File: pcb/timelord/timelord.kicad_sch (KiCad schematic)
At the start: 37 parts, among them J1 GPIO, J2 BCKP_PWR, J3 OLED, J4 EXTERNAL, J5 SMA, J6 SMA, Q1 BC846, Q2 BC846, U1 NEO-F10T, U2 DS3232M

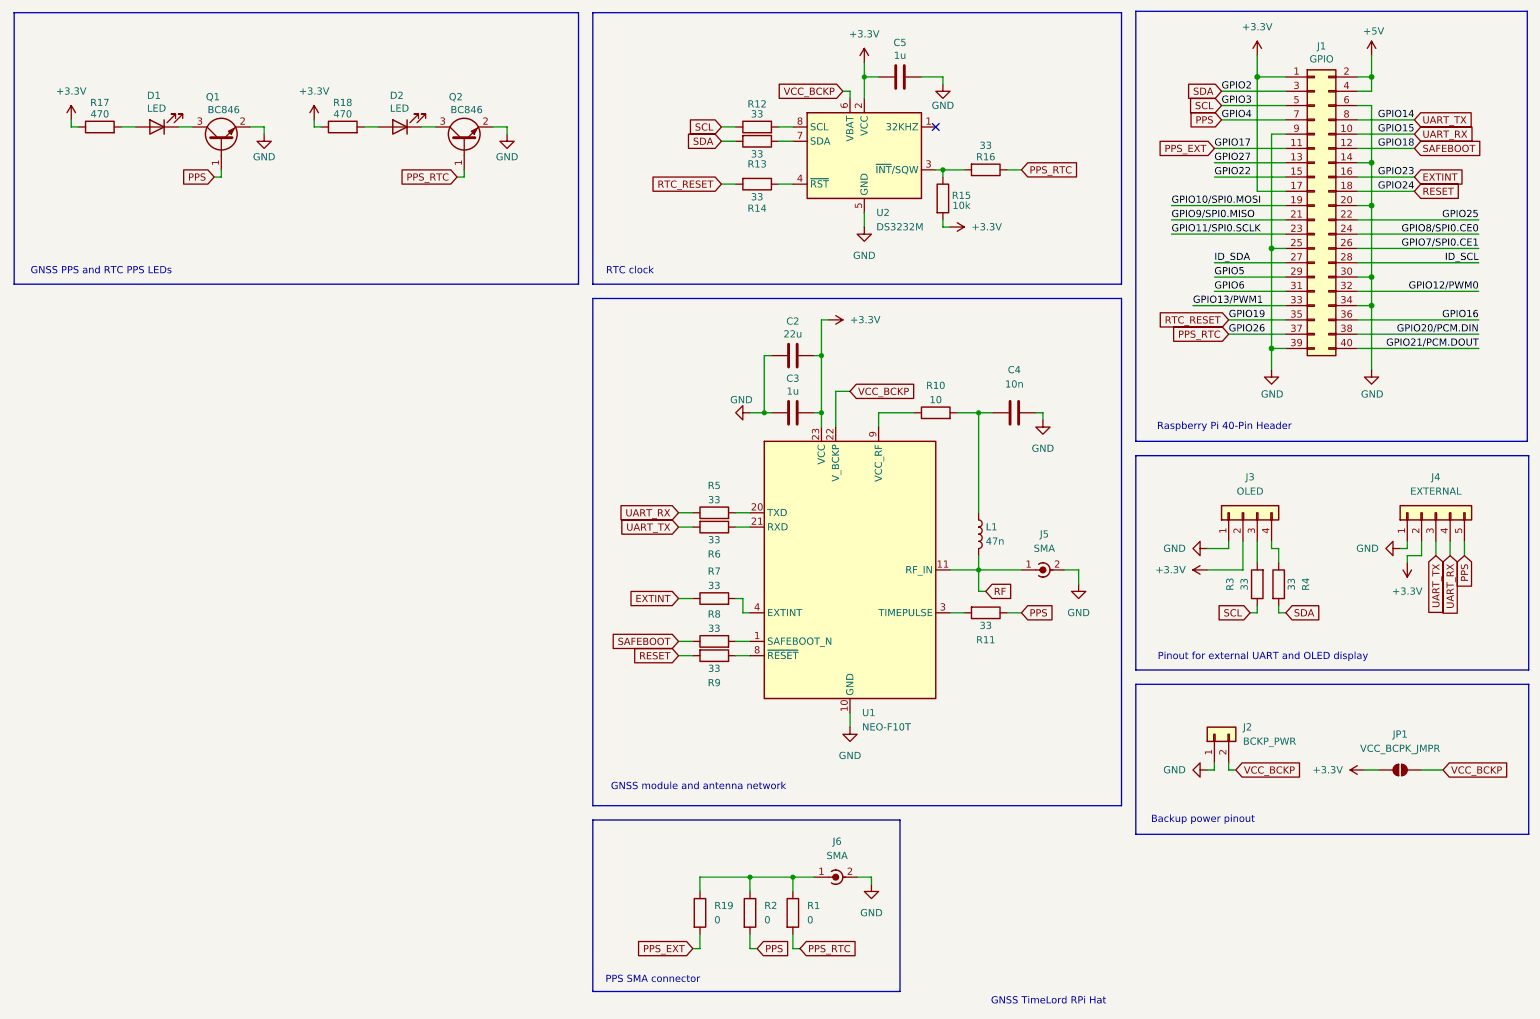
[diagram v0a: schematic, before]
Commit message: Changes
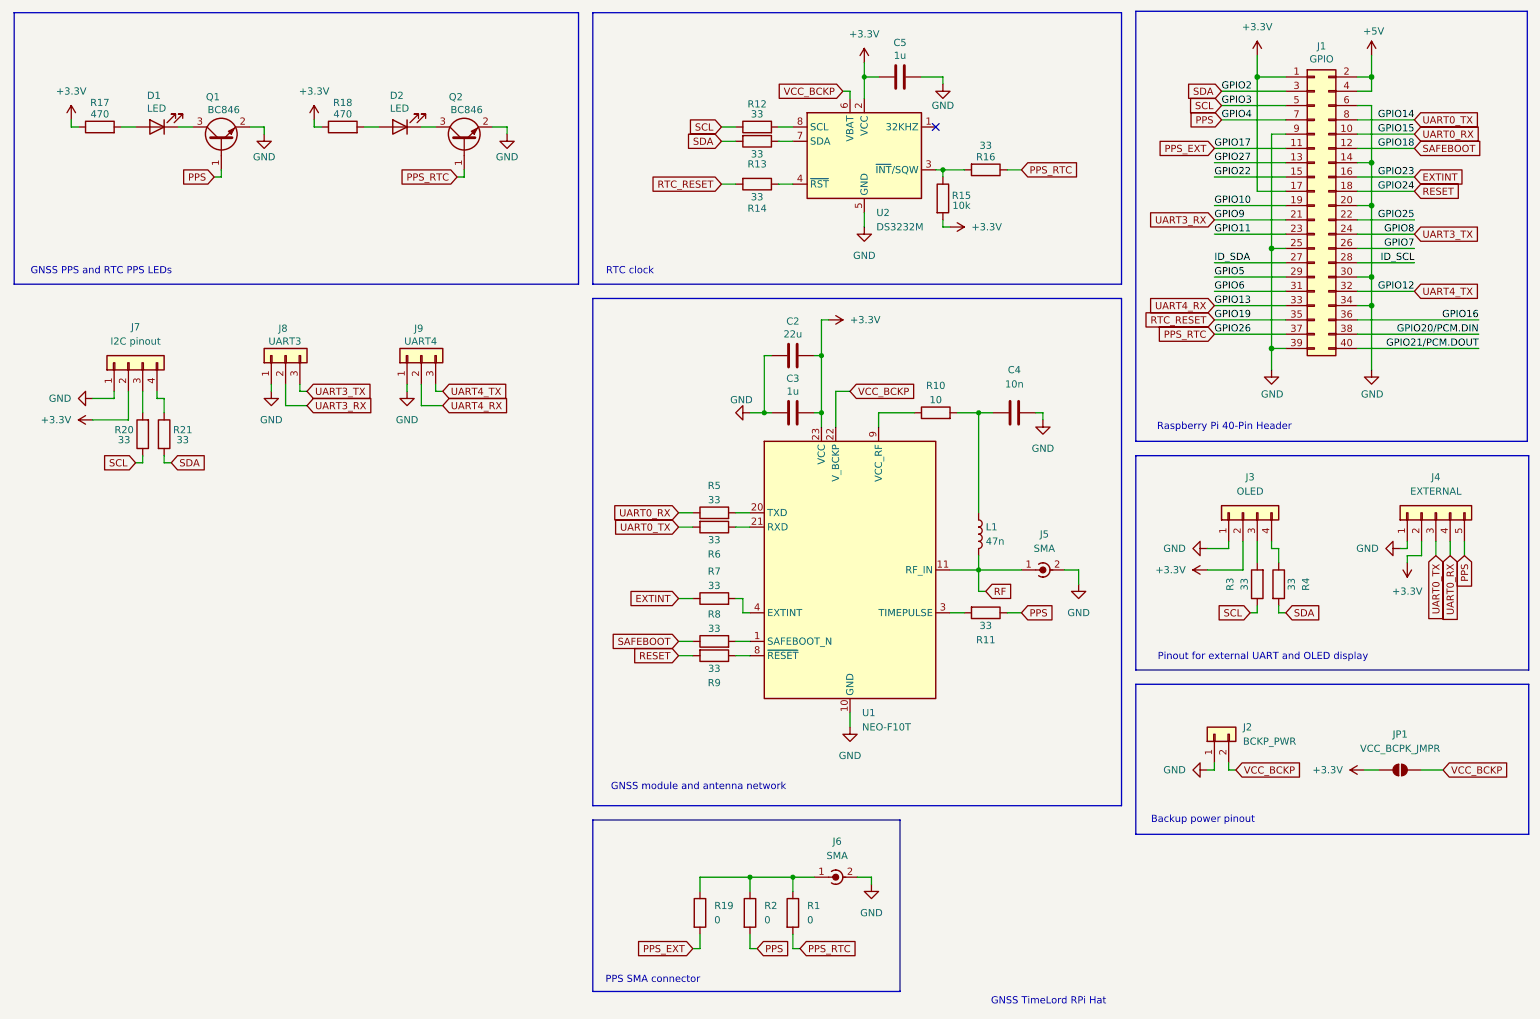
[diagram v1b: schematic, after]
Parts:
- added J7: I2C pinout, Connector_PinSocket_2.54mm:PinSocket_1x04_P2.54mm_Vertical, symbol Connector_Generic:Conn_01x04
- added J8: UART3, Connector_PinHeader_2.54mm:PinHeader_1x03_P2.54mm_Vertical, symbol Connector_Generic:Conn_01x03
- added J9: UART4, Connector_PinHeader_2.54mm:PinHeader_1x03_P2.54mm_Vertical, symbol Connector_Generic:Conn_01x03
- added R20, R21: 33, Resistor_SMD:R_0603_1608Metric, symbol Device:R
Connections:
- net +3.3V: now also J7.2 (Pin_2)
- net GND: now also J7.1 (Pin_1), J8.1 (Pin_1), J9.1 (Pin_1)
- net SCL: now also R20.1
- net SDA: now also R21.2
- net GPIO10/SPI0.MOSI renamed GPIO10
- net GPIO11/SPI0.SCLK renamed GPIO11
- net GPIO12/PWM0 renamed UART4_TX
- net UART4_TX: now also J9.3 (Pin_3)
- net GPIO13/PWM1 renamed UART4_RX
- net UART4_RX: now also J9.2 (Pin_2)
- net GPIO7/SPI0.CE1 renamed GPIO7
- net GPIO8/SPI0.CE0 renamed UART3_TX
- net UART3_TX: now also J8.3 (Pin_3)
- net GPIO9/SPI0.MISO renamed UART3_RX
- net UART3_RX: now also J8.2 (Pin_2)
- net UART_RX renamed UART0_RX
- net UART_TX renamed UART0_TX
- new net: J7.3 (Pin_3), R20.2
- new net: J7.4 (Pin_4), R21.1
